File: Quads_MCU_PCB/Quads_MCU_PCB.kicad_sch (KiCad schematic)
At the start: 84 parts, among them J1 USB_C_Receptacle_USB2.0_16P, J2 Conn_01x06_Pin, J3 Conn_01x02_Pin, J4 Conn_01x03_Pin, J5 Conn_01x03_Pin, J6 Conn_01x03_Pin, J7 Conn_01x03_Pin, SW1 SW_Push, U1 STM32H723ZGTx, U3 ISOW1044, U4 TSR_1-2450, U5 AP7361C-33E, U6 ISOW1044, U7 ISOW1044, U8 MCP2518FD-xQBB, U9 ISOW1044, Y1 40MHz

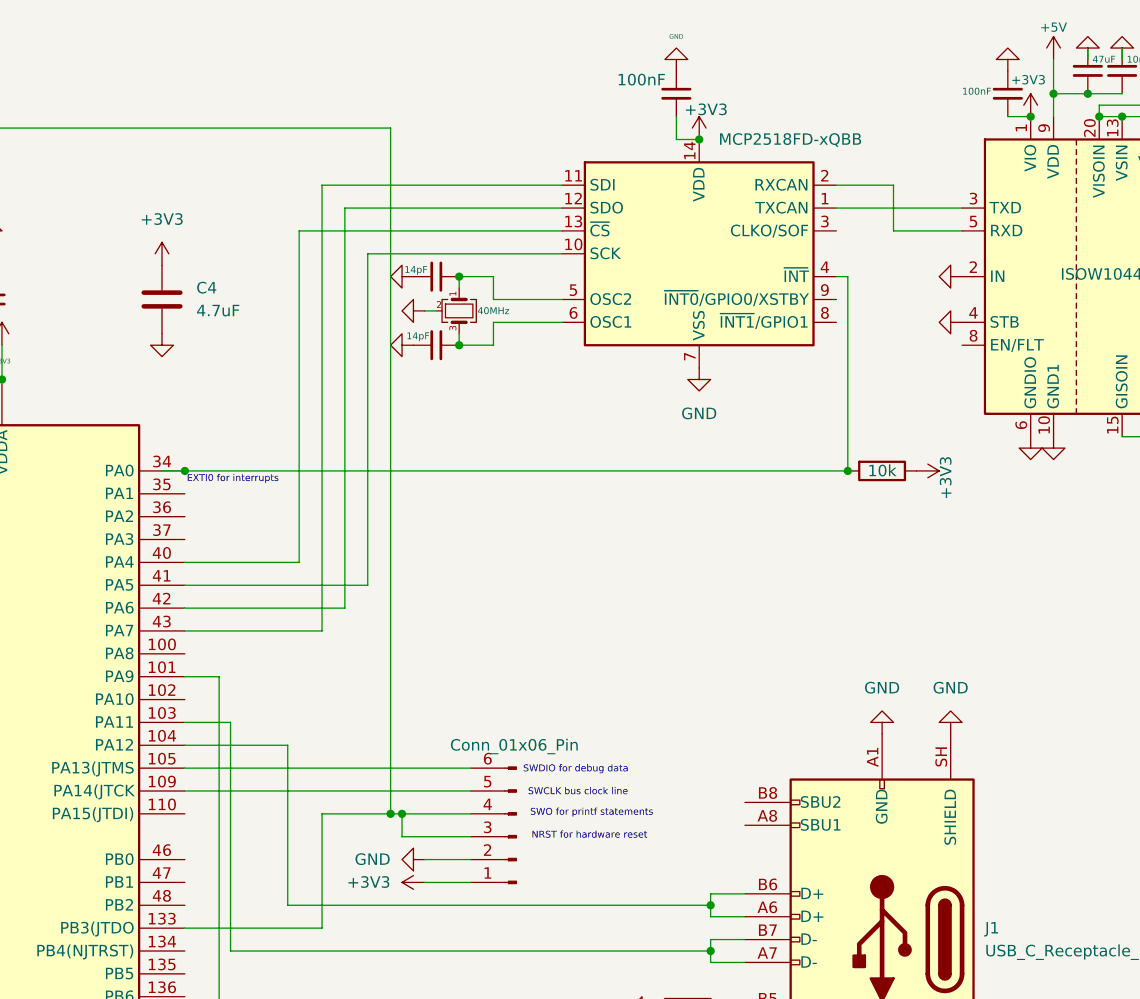
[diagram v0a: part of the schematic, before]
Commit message: Fixed some wiring issues
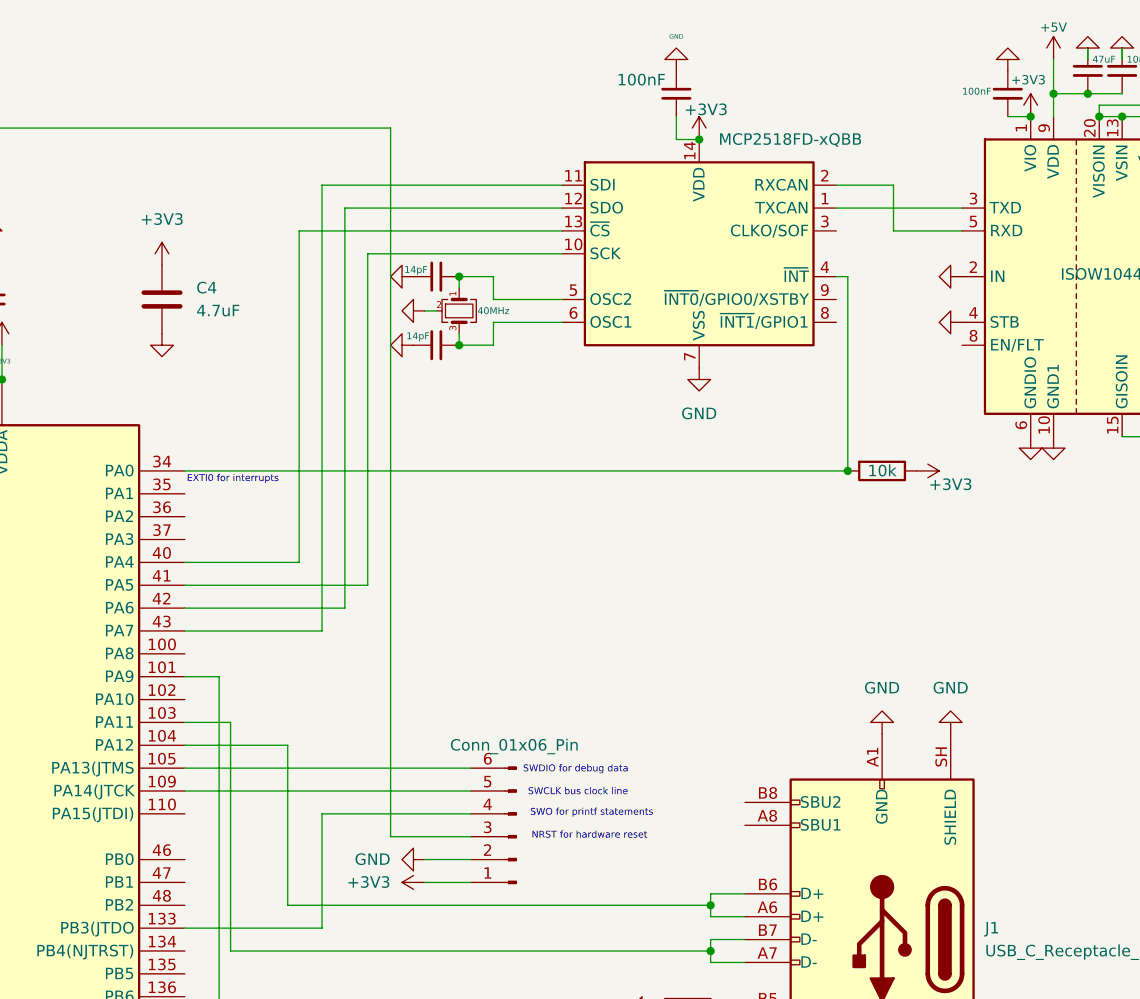
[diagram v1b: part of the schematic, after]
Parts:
- C27, C28, C29, C30, C31, C32, C33, C34, C35, C36, C37, C38, C39, C40, C41, C42, C43, C44, C45, C46, C47, C50, C51, C52, C53, C54, C55, C56: footprint Diode_SMD:Nexperia_DSN1608-2_1.6x0.8mm -> (none)
- D3, D4: footprint Diode_SMD:D_SMA -> (none)
- J3: footprint Connector:Tag-Connect_TC2030-IDC-FP_2x03_P1.27mm_Vertical -> (none)
- J4, J5, J6, J7: footprint Diode_SMD:D_SMF -> (none)
- R10, R11, R13, R9: footprint Package_SO:SOIC-20W_7.5x12.8mm_P1.27mm -> (none)
- SW1: footprint Button_Switch_SMD:Nidec_Copal_CAS-120A -> Button_Switch_SMD:SW_Push_1P1T_NO_E-Switch_TL3301NxxxxxG
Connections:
- net at C1.2, J2.3 (Pin_3), U1.25 (NRST): no longer J2.4 (Pin_4), U1.133 (PB3(JTDO)
- new net: J2.4 (Pin_4), U1.133 (PB3(JTDO)
